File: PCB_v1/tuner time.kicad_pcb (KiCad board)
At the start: 4 copper layers, 80 x 40 mm, 118 parts, among them J1 B6B-PH-K-S, J10 1051640001, J2 B6B-PH-K-S, J3 JST_B2B-XH-A, J4 Conn_01x05_Pin, J5 Conn_01x05_Pin, J6 OLED Conn_02x04, J7 B4B-XH-A, J8 Conn_ARM_JTAG_SWD_10, J9 Conn_01x03, SW1 SW_SPST, SW2 SW_Push, SW3 SW_Push, SW4 SW_Push, SW5 SW_Push, SW6 SW_Push, SW7 SW_Push, SW8 SW_Push, SW9 SW_SPDT, U1 BQ25185DLHR, U2 BQ27441-G1, U3 SMS05T1G, U4 SMS05T1G, U5 DRV8834PWP, U6 STM32F405RGTx, U7 ESD9B5.0ST5G, Y1 Crystal

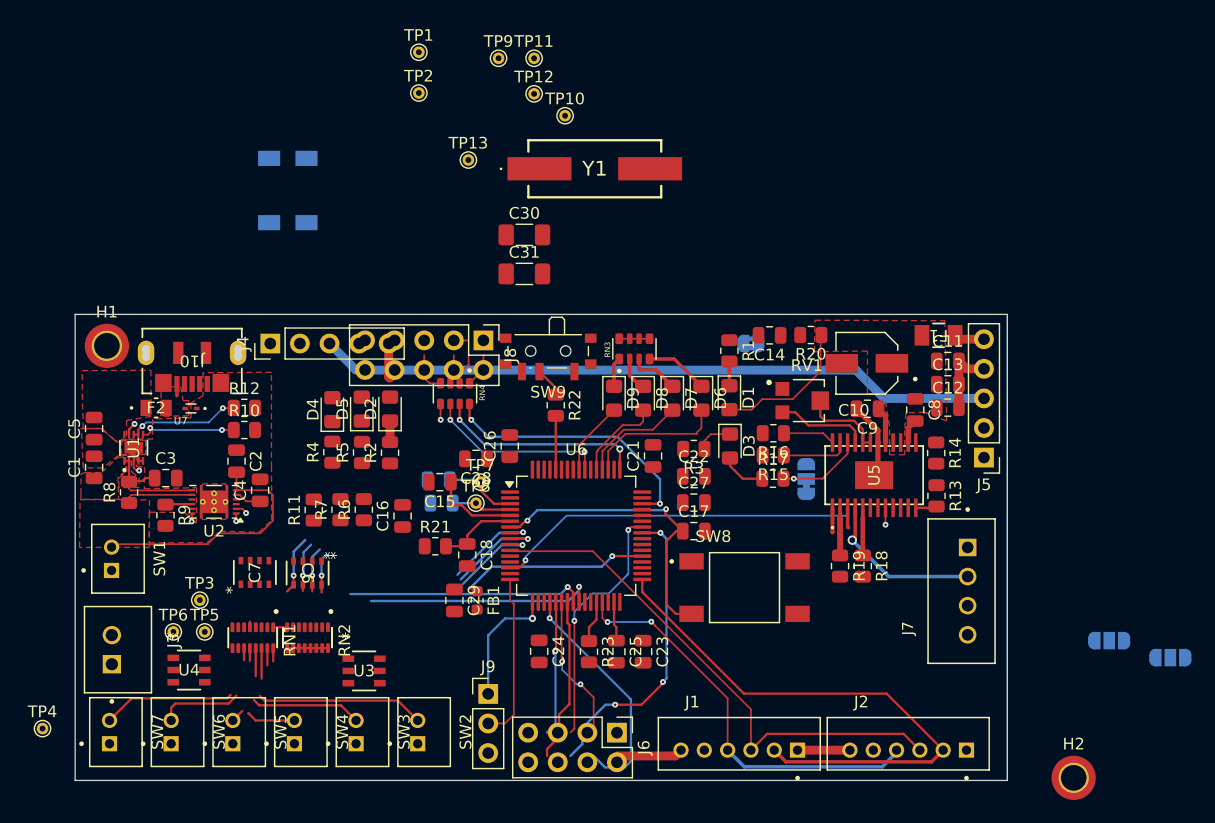
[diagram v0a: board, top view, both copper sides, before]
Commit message: before oscilator
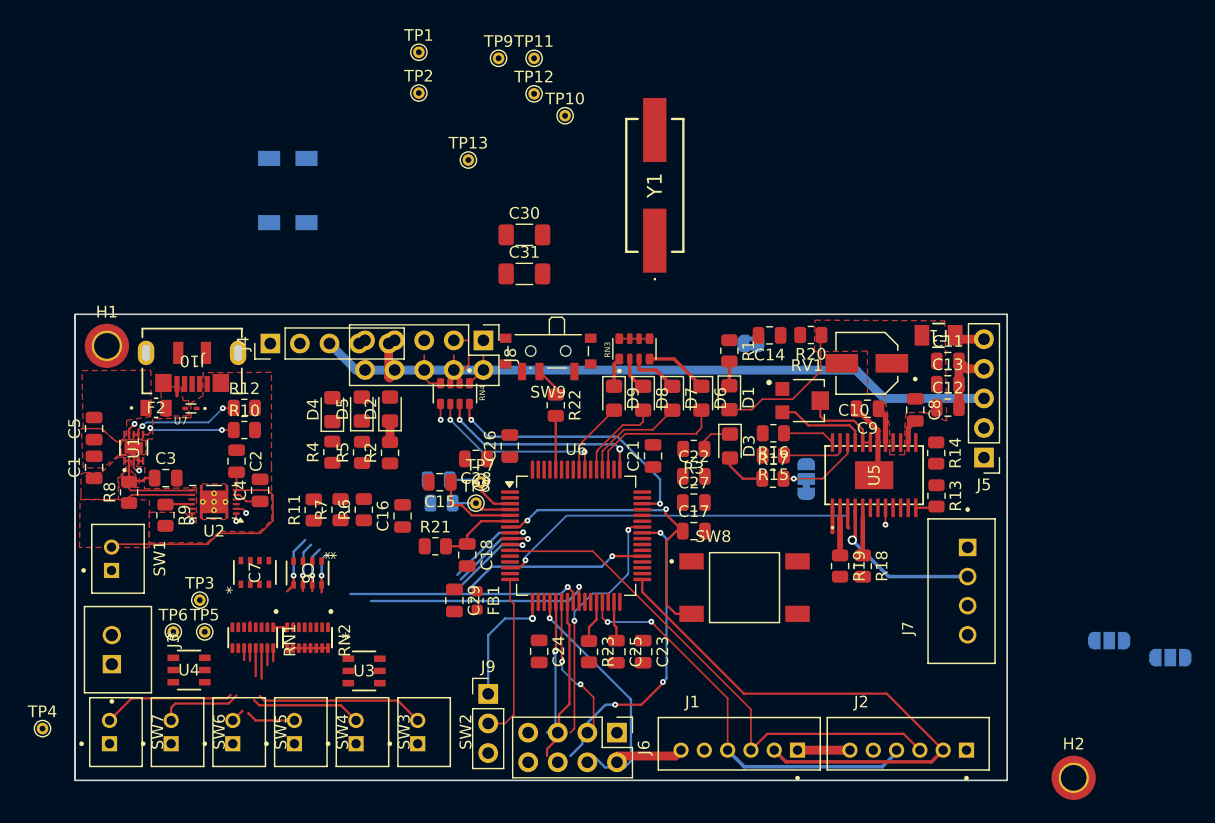
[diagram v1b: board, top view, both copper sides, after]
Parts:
- C1, C11, C12, C13, C14, C15, C16, C17, C18, C19, C2, C20, C21, C22, C23, C24, C25, C26, C27, C28, C29, C3, C4, C5, C8, C9: footprint Capacitor_SMD:C_0805_2012Metric -> C_0805_2012Metric
- C10: footprint Library:CAP_EEE1AA101WR -> CAP_EEE1AA101WR
- C30, C31: footprint Capacitor_SMD:C_1206_3216Metric_Pad1.33x1.80mm_HandSolder -> C_1206_3216Metric_Pad1.33x1.80mm_HandSolder
- C6, C7: footprint GT_library:CAP_CA0612_3P2X1P6_YAG -> CAP_CA0612_3P2X1P6_YAG
- D1, D2, D3, D4, D5, D6, D7, D8, D9: footprint LED_SMD:LED_0805_2012Metric_Pad1.15x1.40mm_HandSolder -> LED_0805_2012Metric_Pad1.15x1.40mm_HandSolder
- F1: footprint Library:C1_BEL -> C1_BEL
- F2: footprint Library:FUS_VISHAY_MFU0805_VIS -> FUS_VISHAY_MFU0805_VIS
- FB1: footprint Inductor_SMD:L_0603_1608Metric -> L_0603_1608Metric
- H1, H2: footprint MountingHole:MountingHole_2.2mm_M2_DIN965_Pad_TopOnly -> MountingHole_2.2mm_M2_DIN965_Pad_TopOnly
- J1, J2: footprint GT_library:JST_B6B-PH-K-S -> JST_B6B-PH-K-S
- J10: footprint Library:CON00906_5_MOL -> CON00906_5_MOL
- J3: footprint Library:JST_B2B-XH-A -> JST_B2B-XH-A
- J4, J5: footprint Connector_PinHeader_2.54mm:PinHeader_1x05_P2.54mm_Vertical -> PinHeader_1x05_P2.54mm_Vertical
- J6: footprint Connector_PinHeader_2.54mm:PinHeader_2x04_P2.54mm_Vertical -> PinHeader_2x04_P2.54mm_Vertical
- J7: footprint Parts_Library:JST_B4B-XH-A -> JST_B4B-XH-A
- J8: footprint Connector_PinHeader_2.54mm:PinHeader_2x05_P2.54mm_Vertical -> PinHeader_2x05_P2.54mm_Vertical
- J9: footprint Connector_PinHeader_2.54mm:PinHeader_1x03_P2.54mm_Vertical -> PinHeader_1x03_P2.54mm_Vertical
- JP1: footprint Jumper:SolderJumper-2_P1.3mm_Bridged2Bar_RoundedPad1.0x1.5mm -> SolderJumper-2_P1.3mm_Bridged2Bar_RoundedPad1.0x1.5mm
- JP2, JP3: footprint Jumper:SolderJumper-3_P1.3mm_Open_RoundedPad1.0x1.5mm -> SolderJumper-3_P1.3mm_Open_RoundedPad1.0x1.5mm
- JP4: footprint Jumper:SolderJumper-3_P1.3mm_Bridged12_RoundedPad1.0x1.5mm -> SolderJumper-3_P1.3mm_Bridged12_RoundedPad1.0x1.5mm
- R1, R10, R11, R12, R13, R14, R15, R16, R17, R18, R19, R2, R20, R21, R22, R23, R3, R4, R5, R6, R7, R8, R9: footprint Resistor_SMD:R_0805_2012Metric -> R_0805_2012Metric
- RN1, RN2: footprint Parts_Library:RESCAXE50P280X160X55-16N -> RESCAXE50P280X160X55-16N
- RN3: footprint Parts_Library:RESCAXS80P320X160X60-8N -> RESCAXS80P320X160X60-8N
- RN4: footprint Parts_Library:RESCAXE80P320X160X70-8N -> RESCAXE80P320X160X70-8N
- RV1: footprint Parts_Library:TRIM_TC33X-2-103E -> TRIM_TC33X-2-103E
- SW1, SW2, SW3, SW4, SW5, SW6, SW7: footprint GT_library:JST_B2B-PH-K-S -> JST_B2B-PH-K-S
- SW8: footprint Library:SW_TS04-66-65-BK-160-SMT -> SW_TS04-66-65-BK-160-SMT
- SW9: footprint Button_Switch_SMD:SW_SPDT_PCM12 -> SW_SPDT_PCM12
- TP1, TP10, TP11, TP12, TP13, TP2, TP3, TP4, TP5, TP6, TP7, TP8, TP9: footprint TestPoint:TestPoint_THTPad_D1.0mm_Drill0.5mm -> TestPoint_THTPad_D1.0mm_Drill0.5mm
- U1: footprint Library:WSON10_DLH_TEX -> WSON10_DLH_TEX
- U2: footprint Package_SON:Texas_S-PDSO-N12 -> Texas_S-PDSO-N12
- U3, U4: footprint Library:SOIC_05T1G_ONS -> SOIC_05T1G_ONS
- U5: footprint Library:SOP65P640X120-25N -> SOP65P640X120-25N
- U6: footprint Package_QFP:LQFP-64_10x10mm_P0.5mm -> LQFP-64_10x10mm_P0.5mm
- U7: footprint Parts_Library:SODFL1006X40N -> SODFL1006X40N
- XTAL1: footprint Parts_Library:SO4_MC-306_SEC -> SO4_MC-306_SEC
- Y1: footprint Library:LFXTAL003237Bulk -> LFXTAL003237Bulk
- moved Y1 5.34 mm to (199.8, 88.9), turned to 90 degrees
